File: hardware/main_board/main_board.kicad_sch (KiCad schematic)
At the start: 80 parts, among them J1 USB_C_Receptacle_USB2.0_16P, J10 Conn_02x05_Counter_Clockwise, J2 UART_DEBUG, J3 BAT1, J6 HV_OUTPUT, J9 Conn_02x05_Counter_Clockwise, Q1 MMBT3904, Q2 MMBT3904, SW1 SW_MEC_5G, U1 MPU-6050, U10 AMS1117, U12 IP5305T, U2 CP2102N-A02-GQFN28, U3 SRV05-4, U4 DFPlayer_mini, U5 ESP32-S3-WROOM1, U6 DS3231MZ, U7 INA3221, U8 BQ27441DRZR-G1A

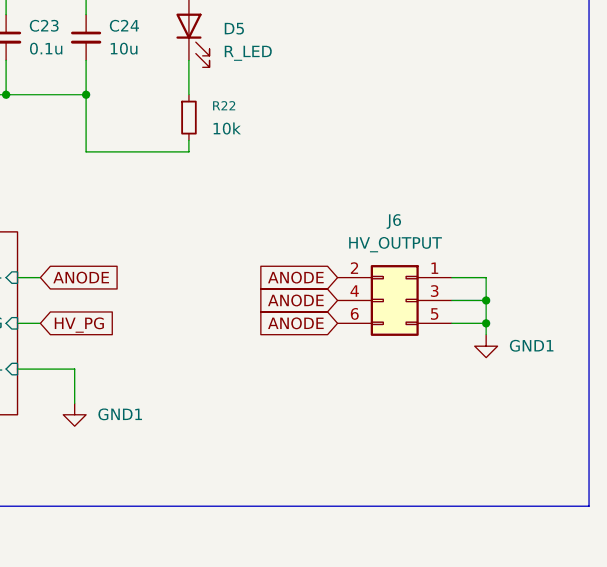
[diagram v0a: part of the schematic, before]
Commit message: WIP(hardware): update in-4 display board
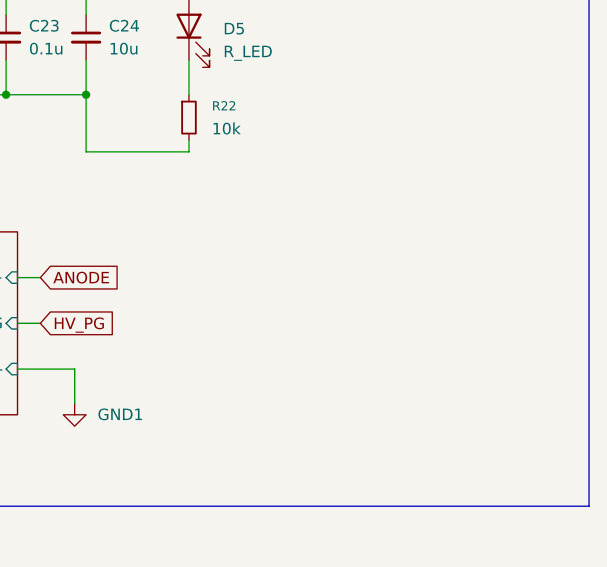
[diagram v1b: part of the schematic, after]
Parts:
- removed J6: HV_OUTPUT, Connector_PinSocket_2.00mm:PinSocket_2x03_P2.00mm_Vertical, symbol Connector_Generic:Conn_02x03_Odd_Even
- J10, J9: footprint (none) -> Connector_PinHeader_2.00mm:PinHeader_2x05_P2.00mm_Vertical
- J2: footprint Connector_PinHeader_2.54mm:PinHeader_1x04_P2.54mm_Horizontal -> Connector_PinHeader_2.00mm:PinHeader_1x04_P2.00mm_Horizontal
